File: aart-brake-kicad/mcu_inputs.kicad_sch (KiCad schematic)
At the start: 0 parts

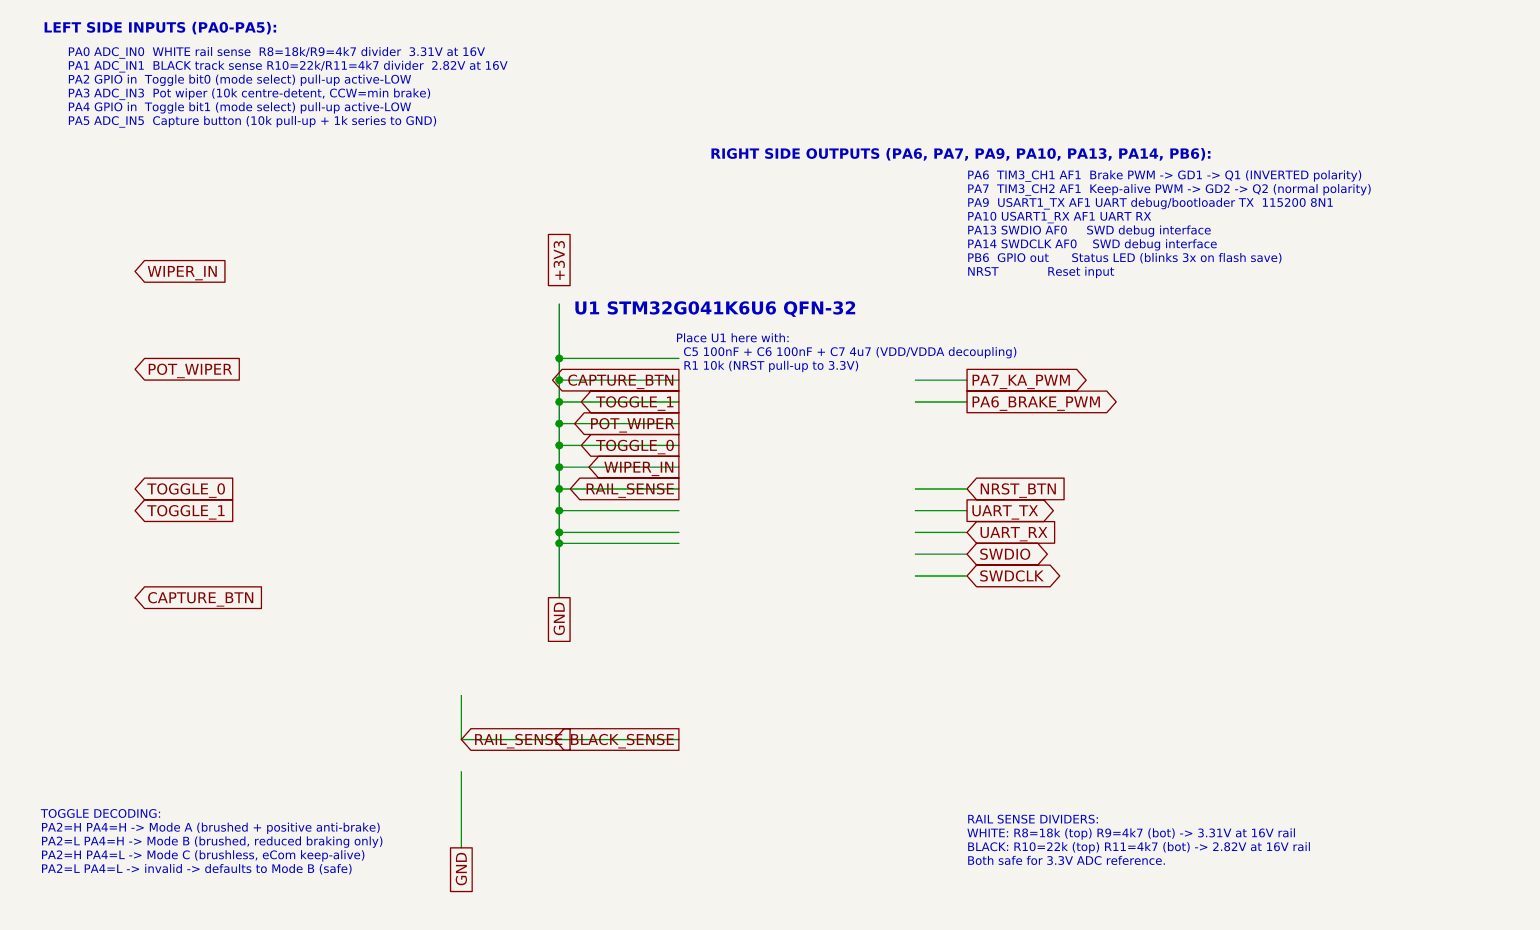
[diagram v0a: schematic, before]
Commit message: Latest doc
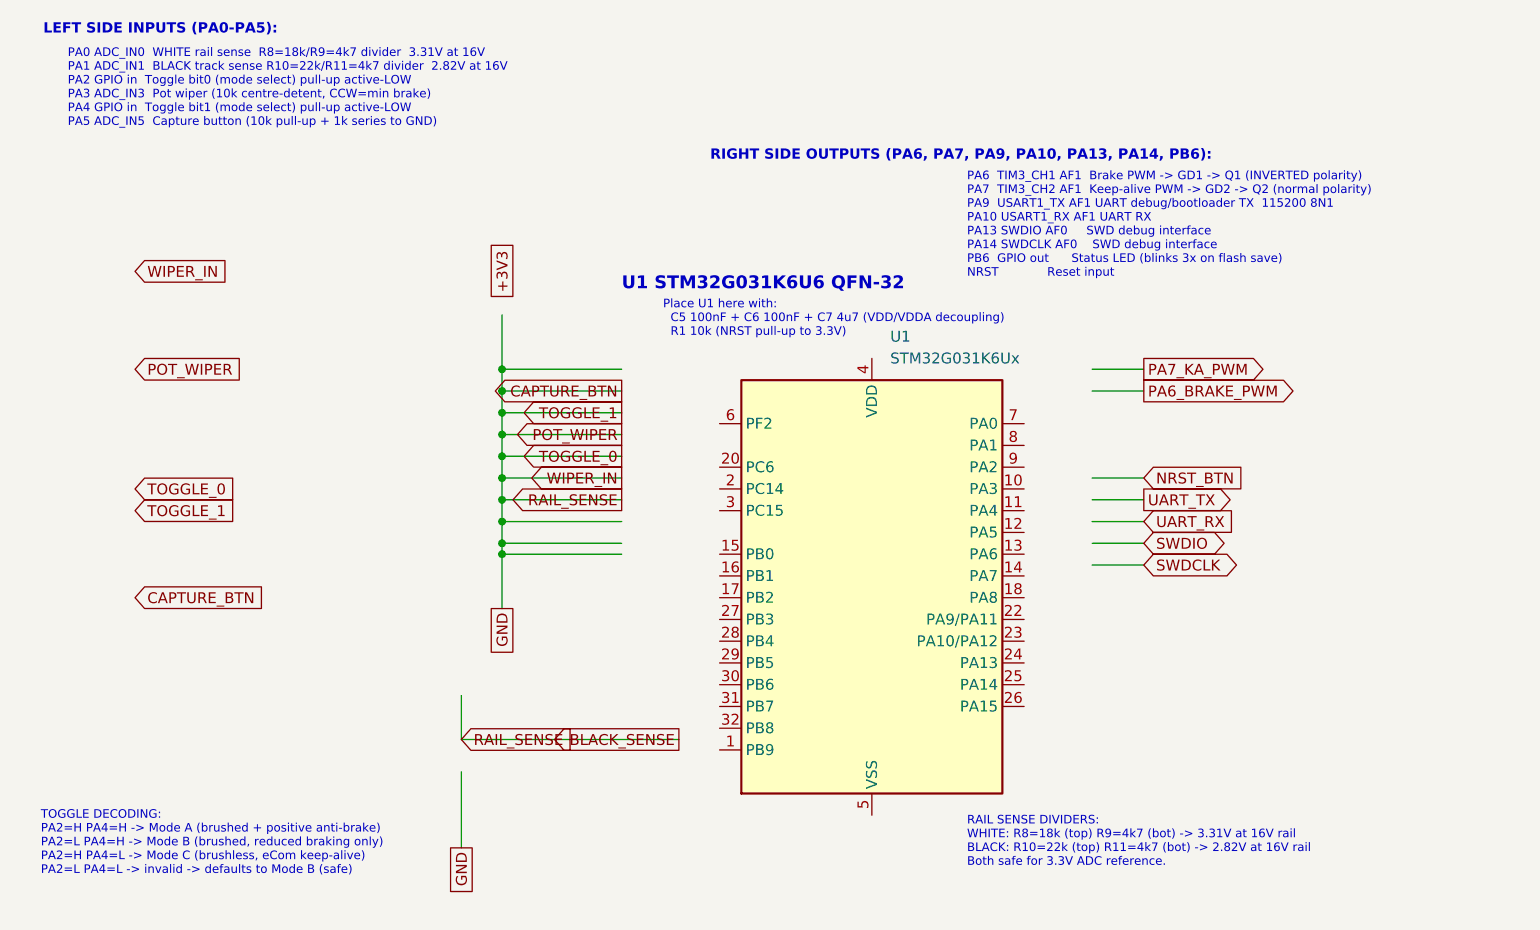
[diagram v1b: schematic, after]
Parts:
- added U1: STM32G031K6Ux, Package_DFN_QFN:QFN-32-1EP_5x5mm_P0.5mm_EP3.45x3.45mm, symbol MCU_ST_STM32G0:STM32G031K6Ux
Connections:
- new net: U1.33 (VSS), U1.5 (VSS)
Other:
- note added: "U1 STM32G031K6U6 QFN-32"
- note removed: "U1 STM32G041K6U6 QFN-32"
